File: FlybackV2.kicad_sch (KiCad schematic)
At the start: 76 parts, among them J1 Conn_01x06, J2 Divisor, J3 Conn_01x03, Q6 2N3906, T2 0399-T208, U1 LT8304, U9 MAX4239

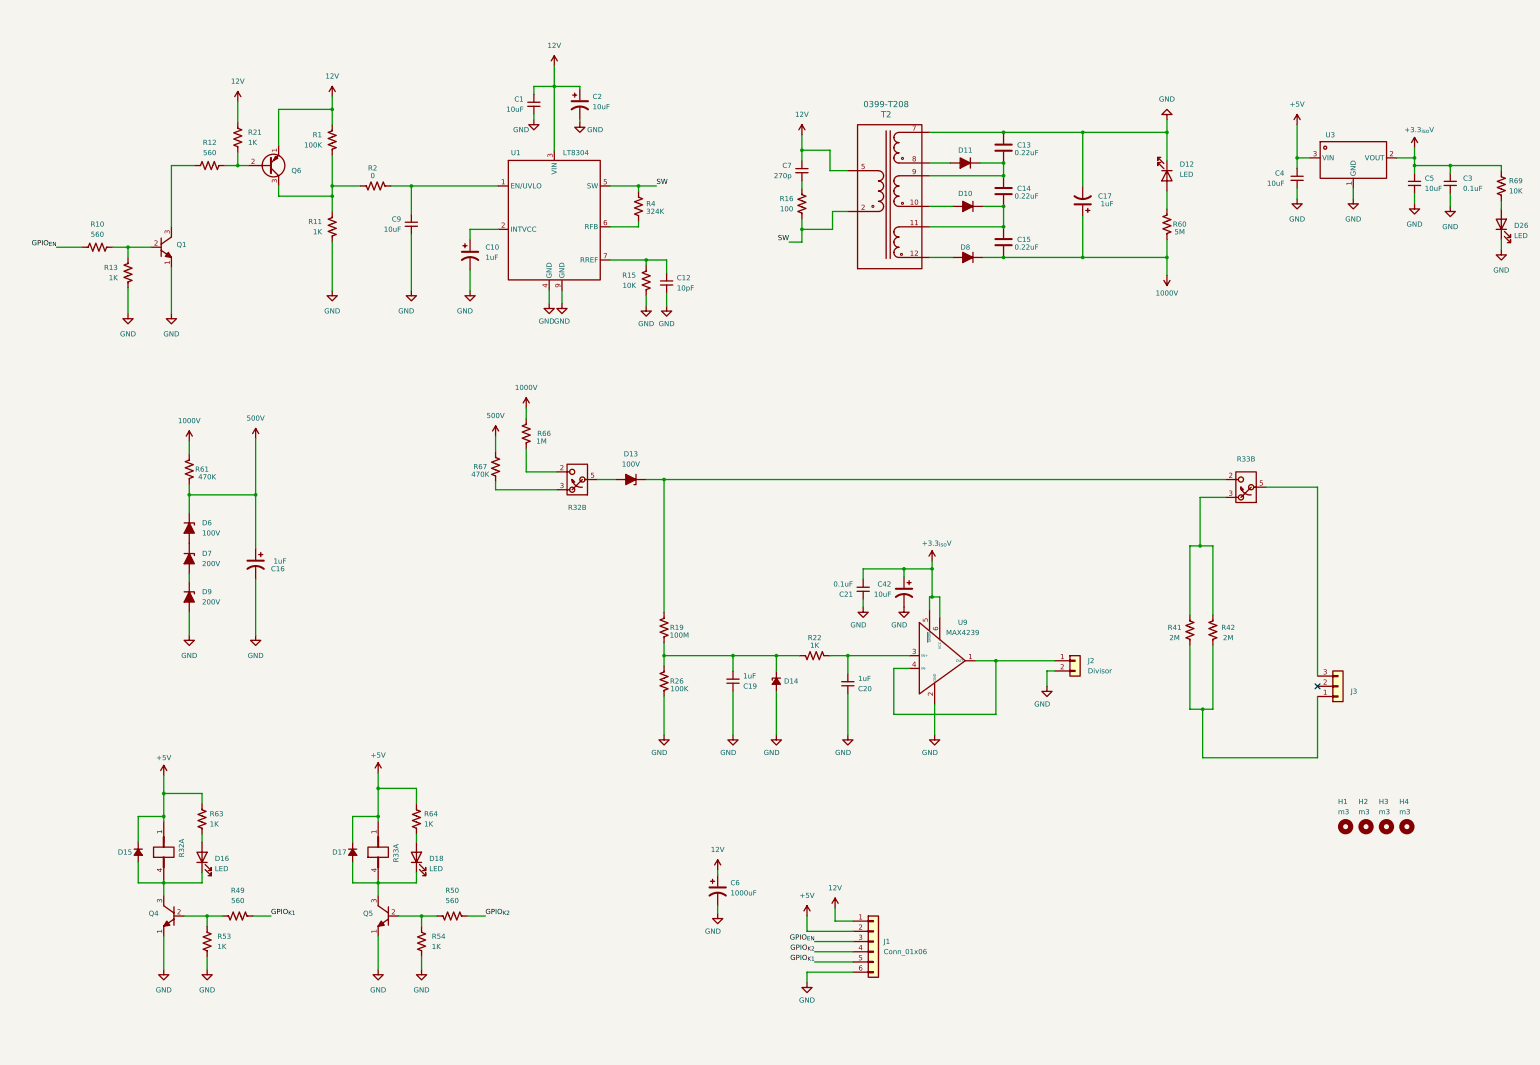
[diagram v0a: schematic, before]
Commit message: update: order in the schematic
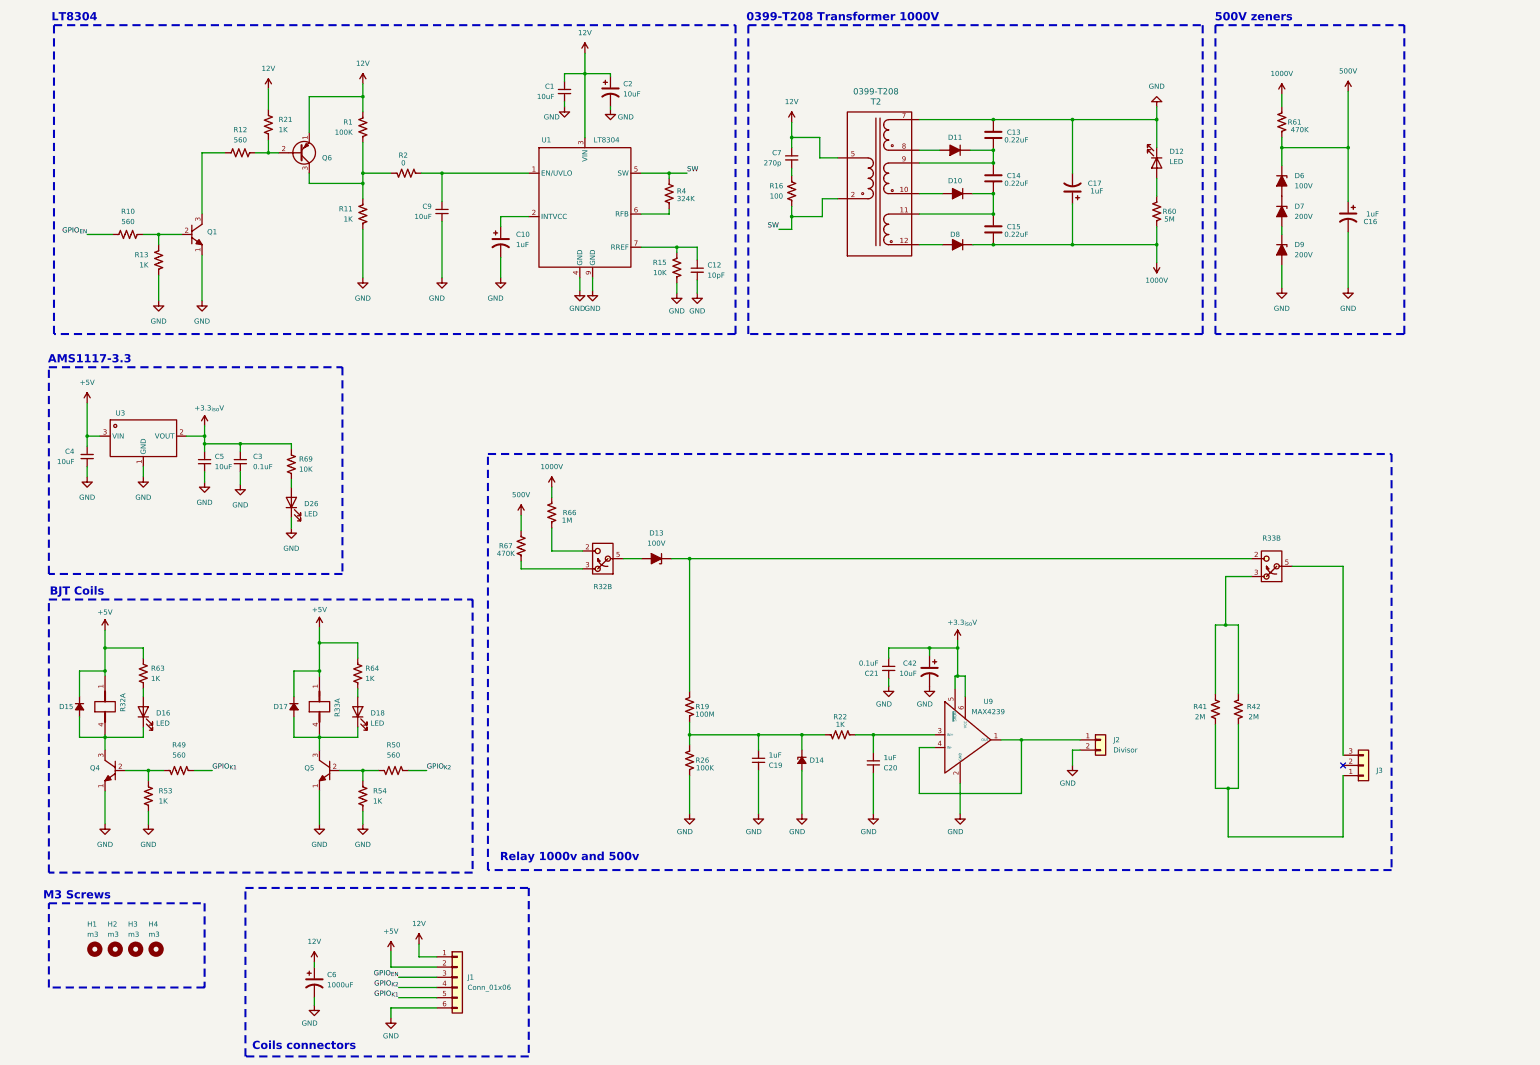
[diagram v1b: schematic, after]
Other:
- note added: "0399-T208 Transformer 1000V"
- note added: "500V zeners"
- note added: "AMS1117-3.3"
- note added: "BJT Coils"
- note added: "Coils connectors"
- note added: "LT8304"
- note added: "M3 Screws"
- note added: "Relay 1000v and 500v"
- moved on the sheet: C1, C10, C12, C13, C14, C15, C16, C17, C19, C2, C20, C21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
